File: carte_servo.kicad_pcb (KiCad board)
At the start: 4 copper layers, 48.4 x 99.2 mm, 157 parts, among them J1 Conn_01x04_Pin, J10 Conn_01x03_Male, J11 Transistor_2, J12 Transistor_1, J13 Transistor_4, J14 Transistor_.3, J16 Conn_01x04_Male, J17 Conn_01x04_Male, J18 Conn_01x03_Male, J19 Conn_01x03_Male, J2 Conn_02x04_Top_Bottom, J24 Conn_LEDs, J25 Conn_AX12, J29 Conn_AX12, J3 Conn_01x04_Pin, J5 Conn_01x03_Male, J6 Conn_01x03_Male, J7 Conn_01x03_Male, J8 Conn_01x03_Male, J9 Conn_01x03_Male, P1 USB_C_Plug_USB2.0, Q1 DMN2011UTS, Q2 DMN2011UTS, Q3 DMN2011UTS, Q4 DMN2011UTS, Q6 DMN2011UTS, Q7 CSD17307Q5A, Q8 CSD17579Q5A, SW2 SW_Push, U1 XGZP6897D_differential_pressu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, U10 TPS563200, U2 XGZP6897D_differential_pressu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, U3 TMC2208_SILENTSTEPSTICK, U4 TMC2208_SILENTSTEPSTICK, U5 74LVC2G241, U6 SN65HVD230, U7 LD1117S33TR_SOT223, U8 ESP32-S3-WROOM-1, U9 LM3150MH

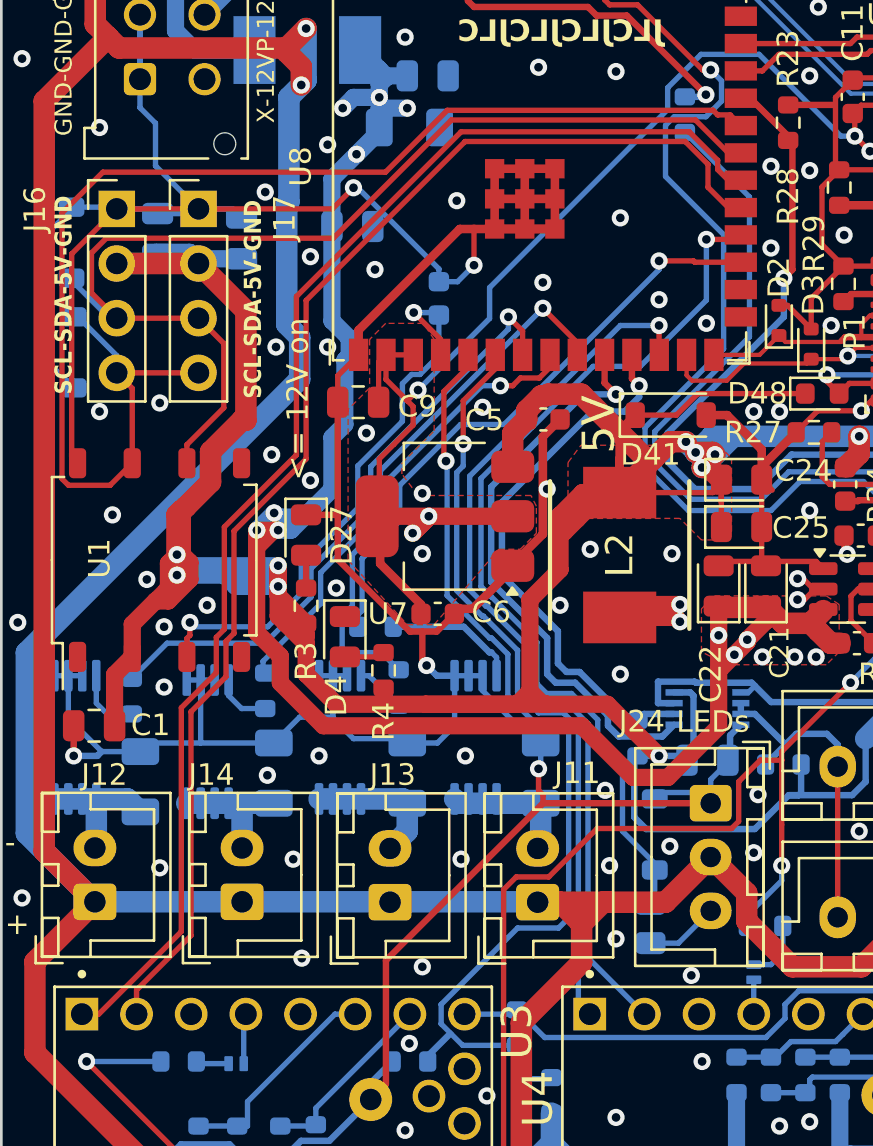
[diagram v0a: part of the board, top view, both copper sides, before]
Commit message: better routing
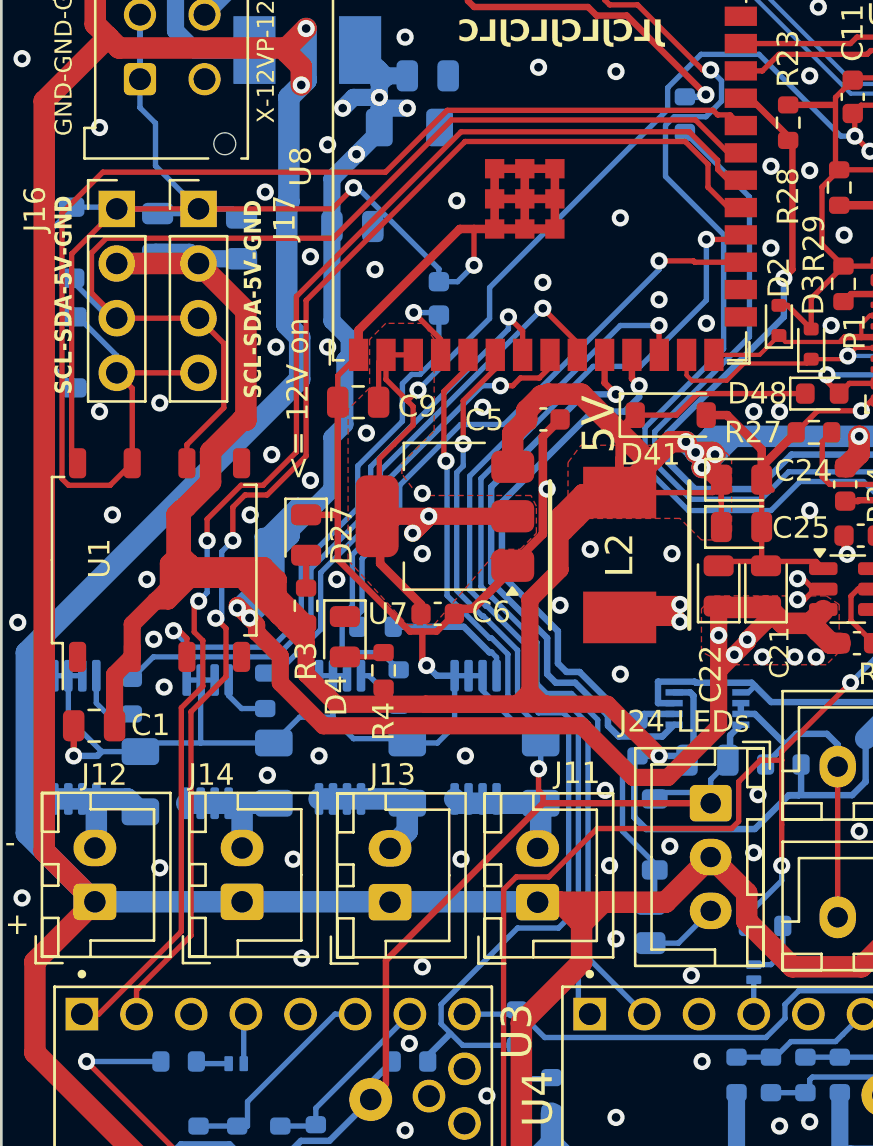
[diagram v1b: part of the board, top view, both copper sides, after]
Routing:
- net 5V: track 340.0 -> 336.5 mm, vias 11 -> 7
- net Pressure_1: track 27.1 -> 29.1 mm
- net STEP_1: track 61.6 -> 63.2 mm, vias 0 -> 2
- net BATT_12V_elec: track 85.3 -> 86.8 mm, vias 13 -> 12
- net DIR_1: track 62.9 -> 63.9 mm, vias 0 -> 2
- net TRANSISTOR_1: track 28.8 -> 29.4 mm
